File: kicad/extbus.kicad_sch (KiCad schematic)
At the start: 19 parts, among them J20 Spare resistors, J21 Power bar, J22 Spare resistors, J23 BUS Slot 2, J24 BUS Slot 1

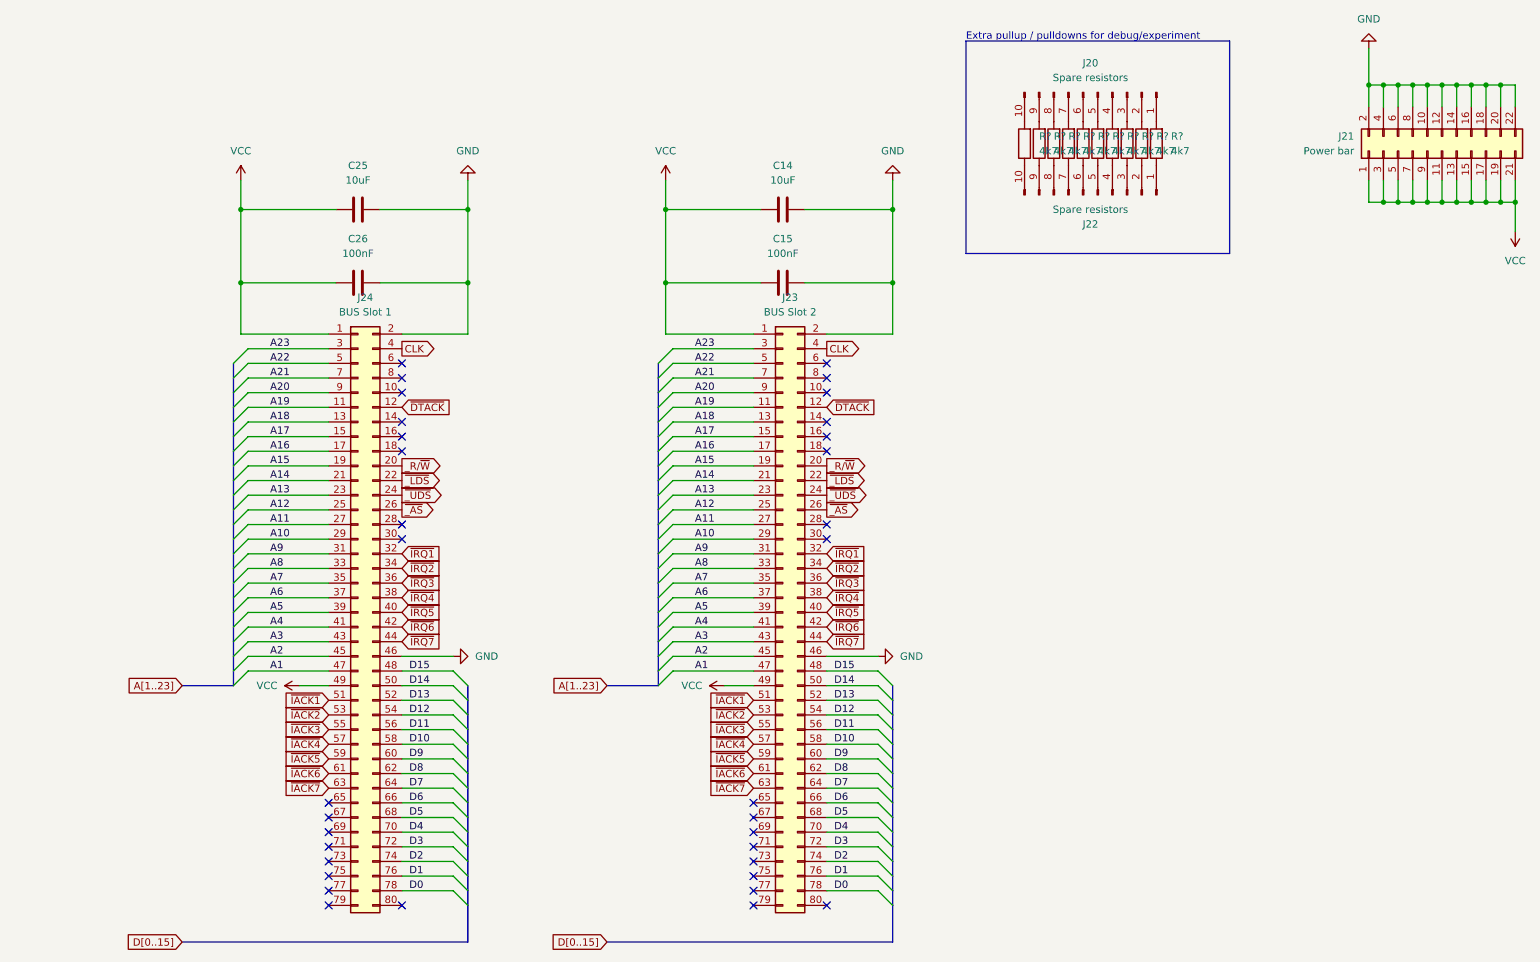
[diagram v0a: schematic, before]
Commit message: saving state
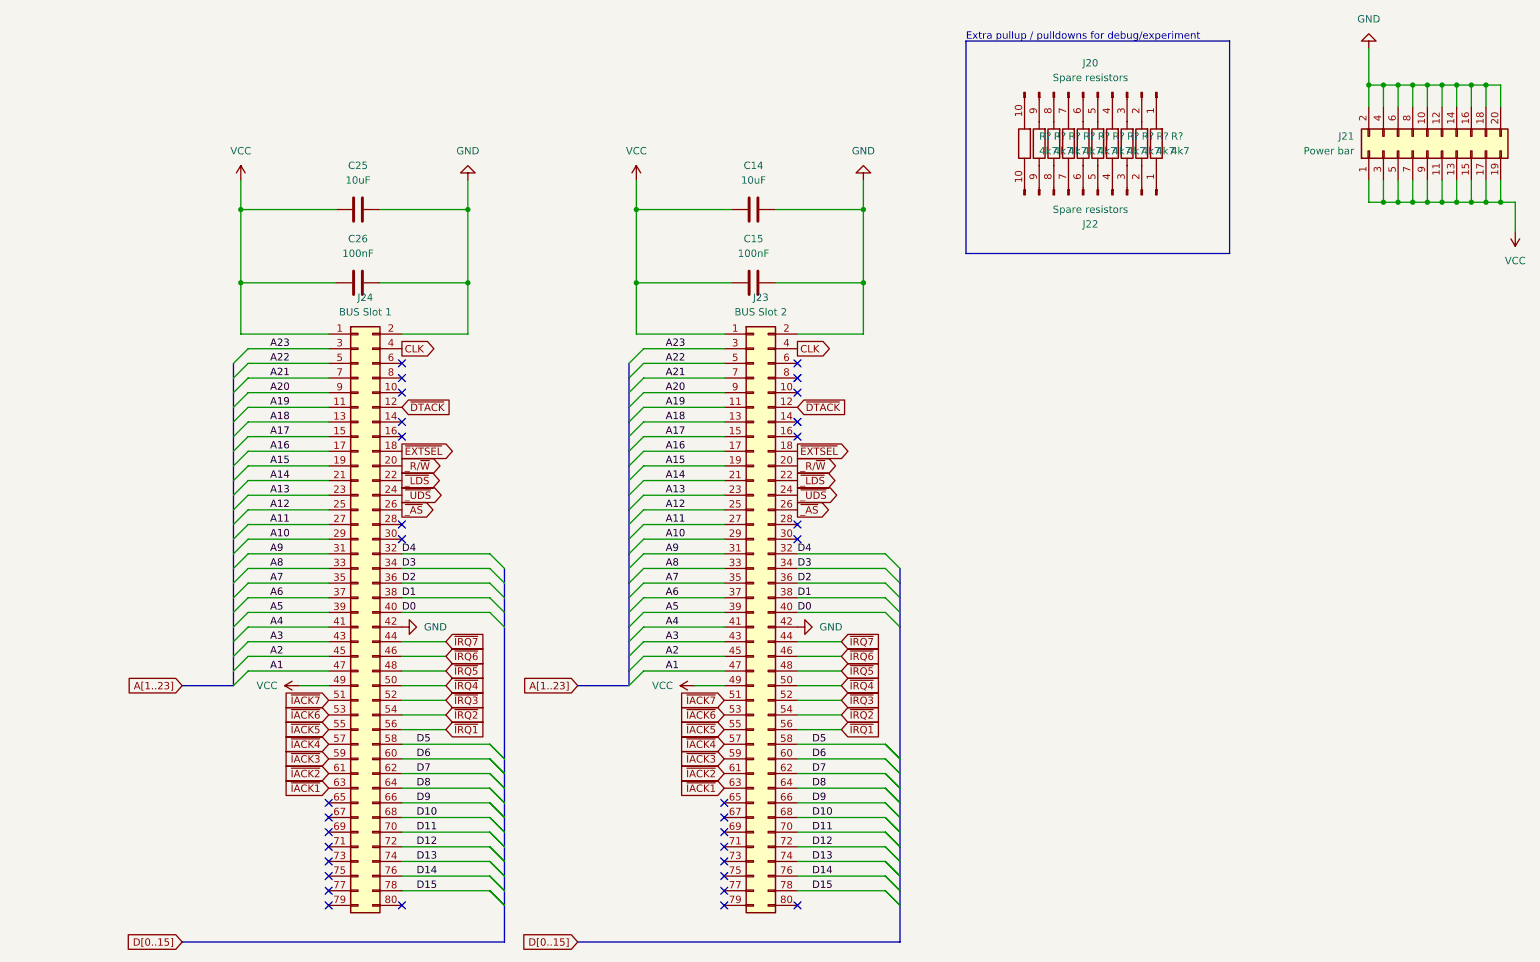
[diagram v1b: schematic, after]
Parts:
- removed J21: Power bar, Connector_PinSocket_2.54mm:PinSocket_2x11_P2.54mm_Vertical, symbol Connector_Generic:Conn_02x11_Odd_Even
- added J21: Power bar, Connector_PinSocket_2.54mm:PinSocket_2x10_P2.54mm_Vertical, symbol Connector_Generic:Conn_02x10_Odd_Even
- C25: footprint Capacitor_THT:CP_Radial_D5.0mm_P2.50mm -> Capacitor_THT:C_Disc_D5.0mm_W2.5mm_P2.50mm
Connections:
- net D0: now also J23.40 (Pin_40), J24.40 (Pin_40); no longer J23.78 (Pin_78), J24.78 (Pin_78)
- net D1: now also J23.38 (Pin_38), J24.38 (Pin_38); no longer J23.76 (Pin_76), J24.76 (Pin_76)
- net D10: now also J23.68 (Pin_68), J24.68 (Pin_68); no longer J23.58 (Pin_58), J24.58 (Pin_58)
- net D11: now also J23.70 (Pin_70), J24.70 (Pin_70); no longer J23.56 (Pin_56), J24.56 (Pin_56)
- net D12: now also J23.72 (Pin_72), J24.72 (Pin_72); no longer J23.54 (Pin_54), J24.54 (Pin_54)
- net D13: now also J23.74 (Pin_74), J24.74 (Pin_74); no longer J23.52 (Pin_52), J24.52 (Pin_52)
- net D14: now also J23.76 (Pin_76), J24.76 (Pin_76); no longer J23.50 (Pin_50), J24.50 (Pin_50)
- net D15: now also J23.78 (Pin_78), J24.78 (Pin_78); no longer J23.48 (Pin_48), J24.48 (Pin_48)
- net D2: now also J23.36 (Pin_36), J24.36 (Pin_36); no longer J23.74 (Pin_74), J24.74 (Pin_74)
- net D3: now also J23.34 (Pin_34), J24.34 (Pin_34); no longer J23.72 (Pin_72), J24.72 (Pin_72)
- net D4: now also J23.32 (Pin_32), J24.32 (Pin_32); no longer J23.70 (Pin_70), J24.70 (Pin_70)
- net D5: now also J23.58 (Pin_58), J24.58 (Pin_58); no longer J23.68 (Pin_68), J24.68 (Pin_68)
- net D6: now also J23.60 (Pin_60), J24.60 (Pin_60); no longer J23.66 (Pin_66), J24.66 (Pin_66)
- net D7: now also J23.62 (Pin_62), J24.62 (Pin_62); no longer J23.64 (Pin_64), J24.64 (Pin_64)
- net D8: now also J23.64 (Pin_64), J24.64 (Pin_64); no longer J23.62 (Pin_62), J24.62 (Pin_62)
- net D9: now also J23.66 (Pin_66), J24.66 (Pin_66); no longer J23.60 (Pin_60), J24.60 (Pin_60)
- net GND: now also J23.42 (Pin_42), J24.42 (Pin_42), J21.10 (Pin_10), J21.12 (Pin_12), J21.14 (Pin_14), J21.16 (Pin_16), J21.18 (Pin_18), J21.2 (Pin_2), J21.20 (Pin_20), J21.4 (Pin_4), J21.6 (Pin_6), J21.8 (Pin_8); no longer J23.46 (Pin_46), J24.46 (Pin_46)
- net VCC: now also J21.1 (Pin_1), J21.11 (Pin_11), J21.13 (Pin_13), J21.15 (Pin_15), J21.17 (Pin_17), J21.19 (Pin_19), J21.3 (Pin_3), J21.5 (Pin_5), J21.7 (Pin_7), J21.9 (Pin_9)
- net ~{IACK1}: now also J23.63 (Pin_63), J24.63 (Pin_63); no longer J23.51 (Pin_51), J24.51 (Pin_51)
- net ~{IACK2}: now also J23.61 (Pin_61), J24.61 (Pin_61); no longer J23.53 (Pin_53), J24.53 (Pin_53)
- net ~{IACK3}: now also J23.59 (Pin_59), J24.59 (Pin_59); no longer J23.55 (Pin_55), J24.55 (Pin_55)
- net ~{IACK5}: now also J23.55 (Pin_55), J24.55 (Pin_55); no longer J23.59 (Pin_59), J24.59 (Pin_59)
- net ~{IACK6}: now also J23.53 (Pin_53), J24.53 (Pin_53); no longer J23.61 (Pin_61), J24.61 (Pin_61)
- net ~{IACK7}: now also J23.51 (Pin_51), J24.51 (Pin_51); no longer J23.63 (Pin_63), J24.63 (Pin_63)
- net ~{IRQ1}: now also J23.56 (Pin_56), J24.56 (Pin_56); no longer J23.32 (Pin_32), J24.32 (Pin_32)
- net ~{IRQ2}: now also J23.54 (Pin_54), J24.54 (Pin_54); no longer J23.34 (Pin_34), J24.34 (Pin_34)
- net ~{IRQ3}: now also J23.52 (Pin_52), J24.52 (Pin_52); no longer J23.36 (Pin_36), J24.36 (Pin_36)
- net ~{IRQ4}: now also J23.50 (Pin_50), J24.50 (Pin_50); no longer J23.38 (Pin_38), J24.38 (Pin_38)
- net ~{IRQ5}: now also J23.48 (Pin_48), J24.48 (Pin_48); no longer J23.40 (Pin_40), J24.40 (Pin_40)
- net ~{IRQ6}: now also J23.46 (Pin_46), J24.46 (Pin_46); no longer J23.42 (Pin_42), J24.42 (Pin_42)
- net ~{EXTSEL}: now reaches J23.18 (Pin_18)
- net ~{EXTSEL}: now also J24.18 (Pin_18)
- no-connect marks 34 -> 32

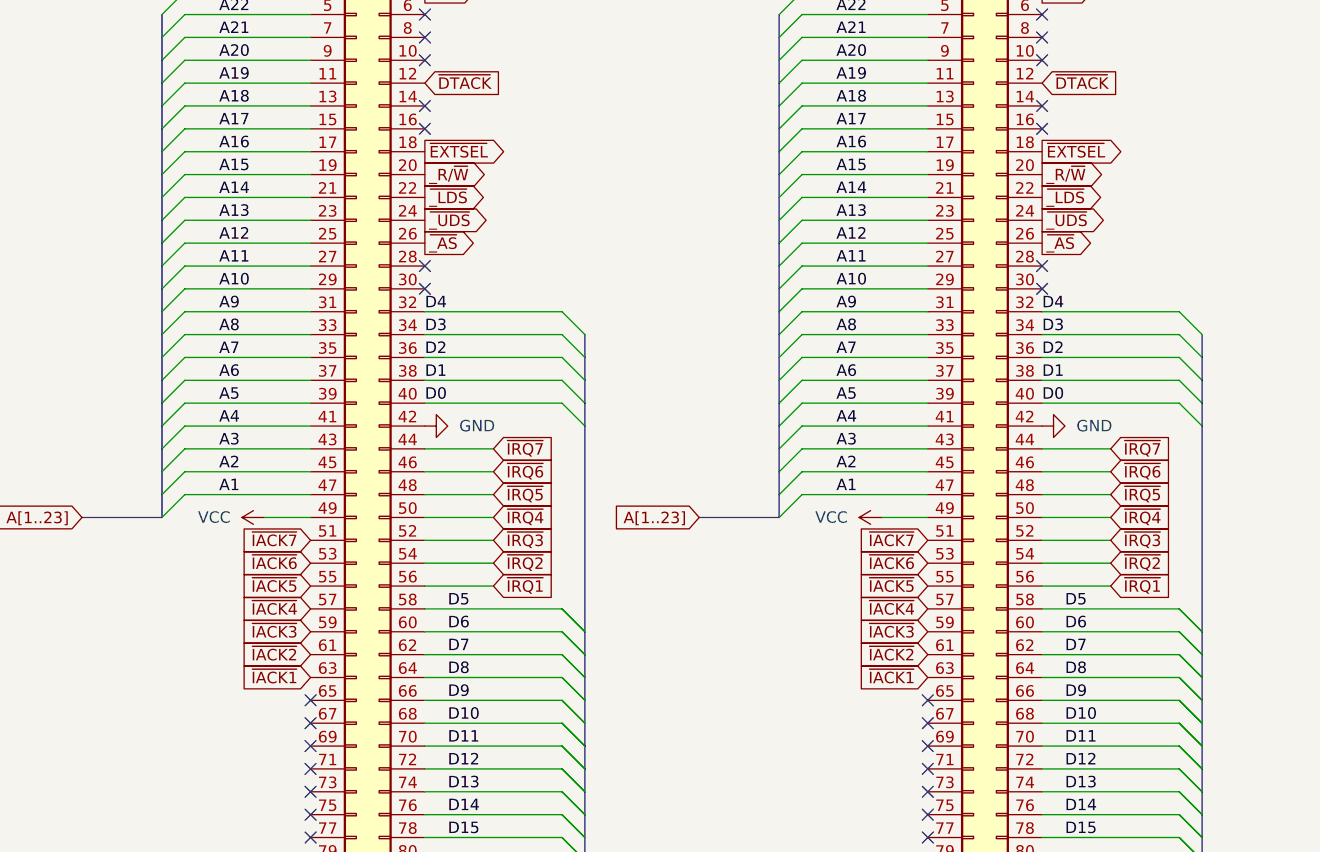
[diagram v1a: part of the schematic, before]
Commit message: saving kicad
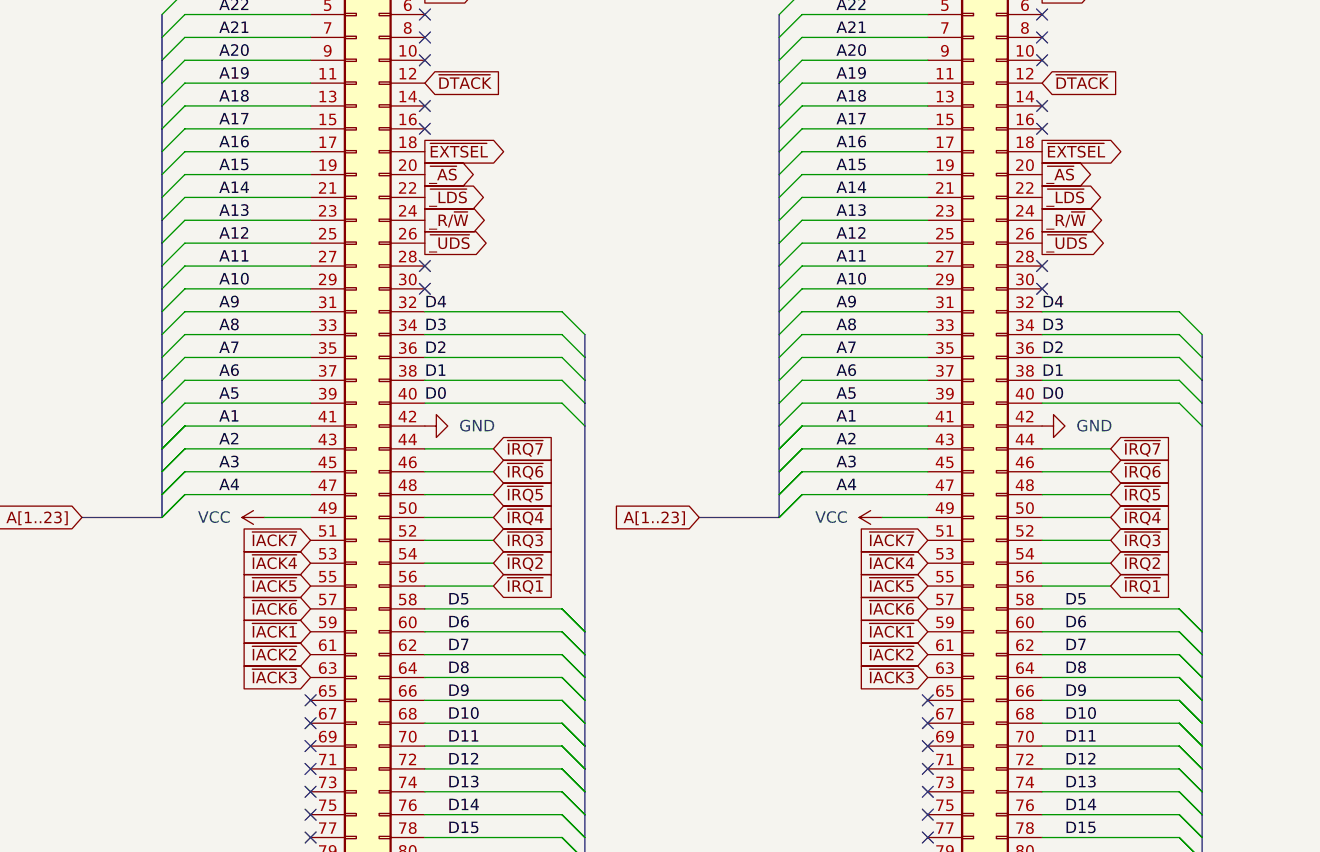
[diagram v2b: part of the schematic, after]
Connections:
- net A1: now also J23.41 (Pin_41), J24.41 (Pin_41); no longer J23.47 (Pin_47), J24.47 (Pin_47)
- net A2: now also J23.43 (Pin_43), J24.43 (Pin_43); no longer J23.45 (Pin_45), J24.45 (Pin_45)
- net A3: now also J23.45 (Pin_45), J24.45 (Pin_45); no longer J23.43 (Pin_43), J24.43 (Pin_43)
- net A4: now also J23.47 (Pin_47), J24.47 (Pin_47); no longer J23.41 (Pin_41), J24.41 (Pin_41)
- net _R/~{W}: now also J23.24 (Pin_24), J24.24 (Pin_24); no longer J23.20 (Pin_20), J24.20 (Pin_20)
- net ~{IACK1}: now also J23.59 (Pin_59), J24.59 (Pin_59); no longer J23.63 (Pin_63), J24.63 (Pin_63)
- net ~{IACK3}: now also J23.63 (Pin_63), J24.63 (Pin_63); no longer J23.59 (Pin_59), J24.59 (Pin_59)
- net ~{IACK4}: now also J23.53 (Pin_53), J24.53 (Pin_53); no longer J23.57 (Pin_57), J24.57 (Pin_57)
- net ~{IACK6}: now also J23.57 (Pin_57), J24.57 (Pin_57); no longer J23.53 (Pin_53), J24.53 (Pin_53)
- net ~{_AS}: now also J23.20 (Pin_20), J24.20 (Pin_20); no longer J23.26 (Pin_26), J24.26 (Pin_26)
- net ~{_UDS}: now also J23.26 (Pin_26), J24.26 (Pin_26); no longer J23.24 (Pin_24), J24.24 (Pin_24)
